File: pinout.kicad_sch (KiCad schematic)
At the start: 1 part

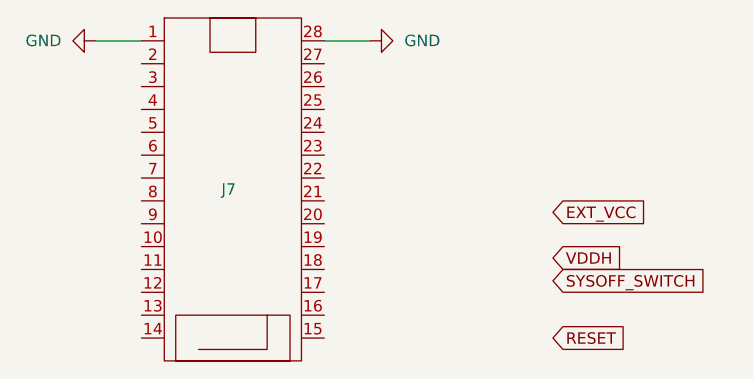
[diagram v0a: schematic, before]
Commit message: Changed Pinout
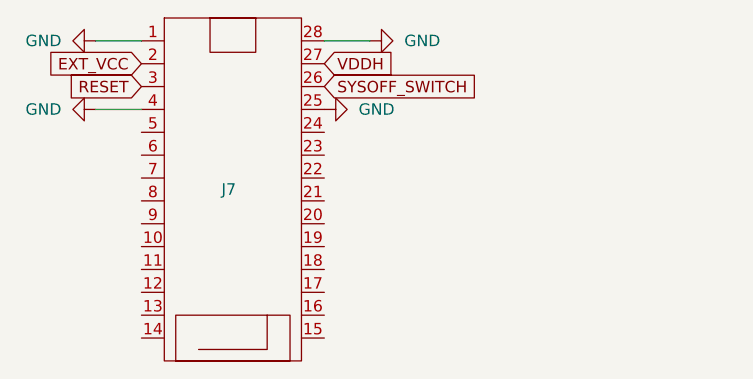
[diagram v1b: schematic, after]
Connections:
- net EXT_VCC: now also J7.2
- net GND: now also J7.25, J7.4
- net RESET: now also J7.3
- net SYSOFF_SWITCH: now also J7.26
- net VDDH: now also J7.27
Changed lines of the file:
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@@
+	(wire
+		(pts
+			(xy 106.68 85.09) (xy 111.76 85.09)
+		)
+		(stroke
+			(width 0)
+			(type default)
+		)
+	)
 	(wire
 		(pts
@@
 	(global_label "EXT_VCC"
 		(shape input)
-		(at 157.48 96.52 0)
+		(at 111.76 80.01 180)
 		(fields_autoplaced yes)
 		(effects
@@
 				(size 1.27 1.27)
 			)
-			(justify left)
+			(justify right)
 		)
 		(property "Intersheetrefs" "${INTERSHEET_REFS}"
-			(at 168.3875 96.52 0)
-			(effects
-				(font
-					(size 1.27 1.27)
-				)
-				(justify left)
+			(at 100.8525 80.01 0)
+			(effects
+				(font
+					(size 1.27 1.27)
+				)
+				(justify right)
 				(hide yes)
 			)
@@
 	(global_label "SYSOFF_SWITCH"
 		(shape input)
-		(at 157.48 104.14 0)
+		(at 132.08 82.55 0)
 		(fields_autoplaced yes)
 		(effects
@@
 		)
 		(property "Intersheetrefs" "${INTERSHEET_REFS}"
-			(at 175.2819 104.14 0)
+			(at 149.8819 82.55 0)
 			(effects
 				(font
@@
 	(global_label "VDDH"
 		(shape input)
-		(at 157.48 101.6 0)
+		(at 132.08 80.01 0)
 		(fields_autoplaced yes)
 		(effects
@@
 		)
 		(property "Intersheetrefs" "${INTERSHEET_REFS}"
-			(at 165.4243 101.6 0)
+			(at 140.0243 80.01 0)
 			(effects
 				(font
@@
 	(global_label "RESET"
 		(shape input)
-		(at 157.48 110.49 0)
+		(at 111.76 82.55 180)
 		(fields_autoplaced yes)
 		(effects
@@
 				(size 1.27 1.27)
 			)
-			(justify left)
+			(justify right)
 		)
 		(property "Intersheetrefs" "${INTERSHEET_REFS}"
-			(at 166.2103 110.49 0)
-			(effects
-				(font
-					(size 1.27 1.27)
-				)
-				(justify left)
+			(at 103.0297 82.55 0)
+			(effects
+				(font
+					(size 1.27 1.27)
+				)
+				(justify right)
 				(hide yes)
 			)
@@
 	(symbol
 		(lib_id "power:GND")
+		(at 106.68 85.09 270)
+		(unit 1)
+		(exclude_from_sim no)
+		(in_bom yes)
+		(on_board yes)
+		(dnp no)
+		(fields_autoplaced yes)
+		(property "Reference" "#PWR041"
+			(at 100.33 85.09 0)
+			(effects
+				(font
+					(size 1.27 1.27)
+				)
+				(hide yes)
+			)
+		)
+		(property "Value" "GND"
+			(at 102.87 85.0899 90)
+			(effects
+				(font
+					(size 1.27 1.27)
+				)
+				(justify right)
+			)
+		)
+		(property "Footprint" ""
+			(at 106.68 85.09 0)
+			(effects
+				(font
+					(size 1.27 1.27)
+				)
+				(hide yes)
+			)
+		)
+		(property "Datasheet" ""
+			(at 106.68 85.09 0)
+			(effects
+				(font
+					(size 1.27 1.27)
+				)
+				(hide yes)
+			)
+		)
+		(property "Description" "Power symbol creates a global label with name \"GND\" , ground"
+			(at 106.68 85.09 0)
+			(effects
+				(font
+					(size 1.27 1.27)
+				)
+				(hide yes)
+			)
+		)
+		(pin "1"
+		)
+		(instances
+			(project "Slim Keyboard"
+				(path "/5d65a0d4-45a3-4af0-996a-c0381d04499a/f42a8a8a-4a34-440a-8e58-9c442fe0d23e/302a6436-4e3c-4497-ba91-0be99fe995f0"
+					(reference "#PWR041")
+					(unit 1)
+				)
+			)
+		)
+	)
+	(symbol
+		(lib_id "power:GND")
 		(at 106.68 77.47 270)
 		(unit 1)
@@
 					(unit 1)
 				)
+			)
+		)
+	)
+	(symbol
+		(lib_id "power:GND")
+		(at 132.08 85.09 90)
+		(unit 1)
+		(exclude_from_sim no)
+		(in_bom yes)
+		(on_board yes)
+		(dnp no)
+		(fields_autoplaced yes)
+		(property "Reference" "#PWR042"
+			(at 138.43 85.09 0)
+			(effects
+				(font
+					(size 1.27 1.27)
+				)
+				(hide yes)
+			)
+		)
+		(property "Value" "GND"
+			(at 135.89 85.0899 90)
+			(effects
+				(font
+					(size 1.27 1.27)
+				)
+				(justify right)
+			)
+		)
+		(property "Footprint" ""
+			(at 132.08 85.09 0)
+			(effects
+				(font
+					(size 1.27 1.27)
+				)
+				(hide yes)
+			)
+		)
+		(property "Datasheet" ""
+			(at 132.08 85.09 0)
+			(effects
+				(font
+					(size 1.27 1.27)
+				)
+				(hide yes)
+			)
+		)
+		(property "Description" "Power symbol creates a global label with name \"GND\" , ground"
+			(at 132.08 85.09 0)
+			(effects
+				(font
+					(size 1.27 1.27)
+				)
+				(hide yes)
+			)
+		)
+		(pin "1"
+		)
+		(instances
+			(project "Slim Keyboard"
+				(path "/5d65a0d4-45a3-4af0-996a-c0381d04499a/f42a8a8a-4a34-440a-8e58-9c442fe0d23e/302a6436-4e3c-4497-ba91-0be99fe995f0"
+					(reference "#PWR042")
+					(unit 1)
+				)
